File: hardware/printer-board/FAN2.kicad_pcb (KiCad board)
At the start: 2 copper layers, 8 parts, among them J35 TO FAN2, Q6 D882

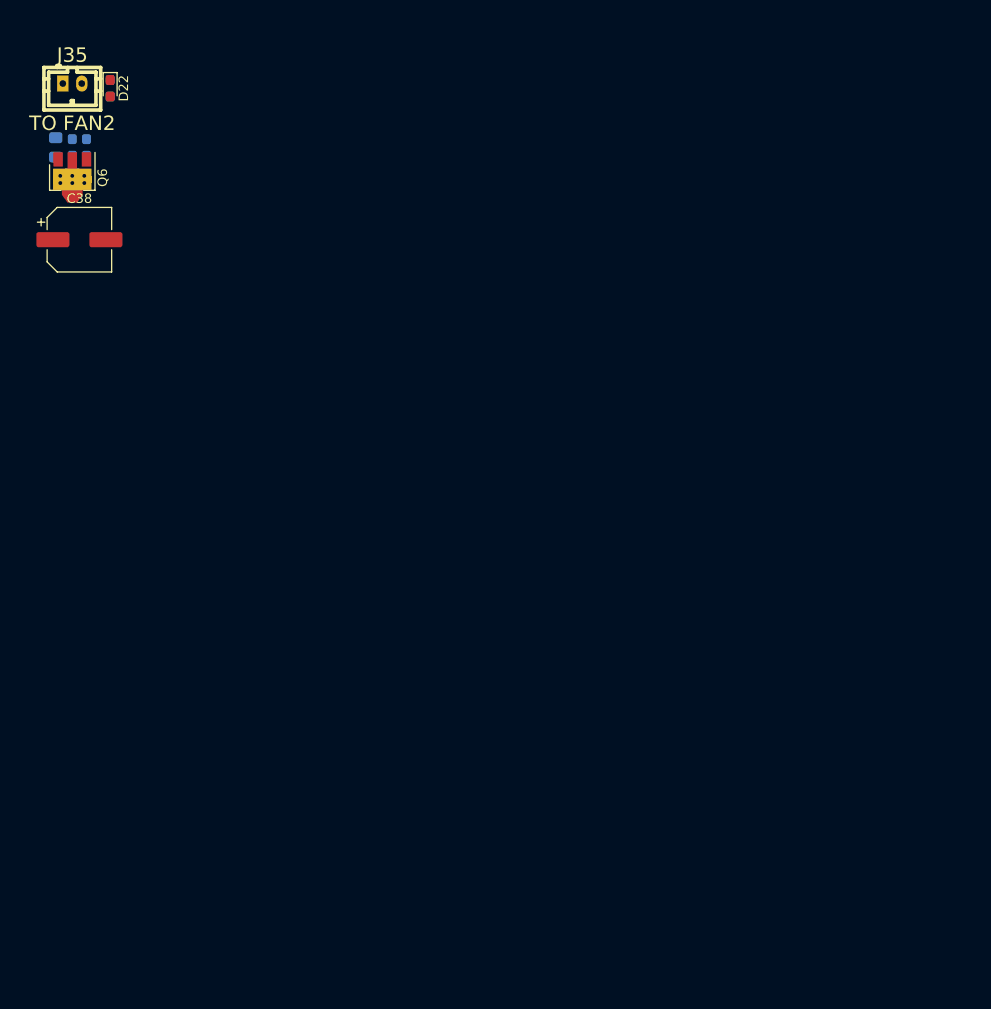
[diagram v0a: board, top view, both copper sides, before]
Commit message: update,
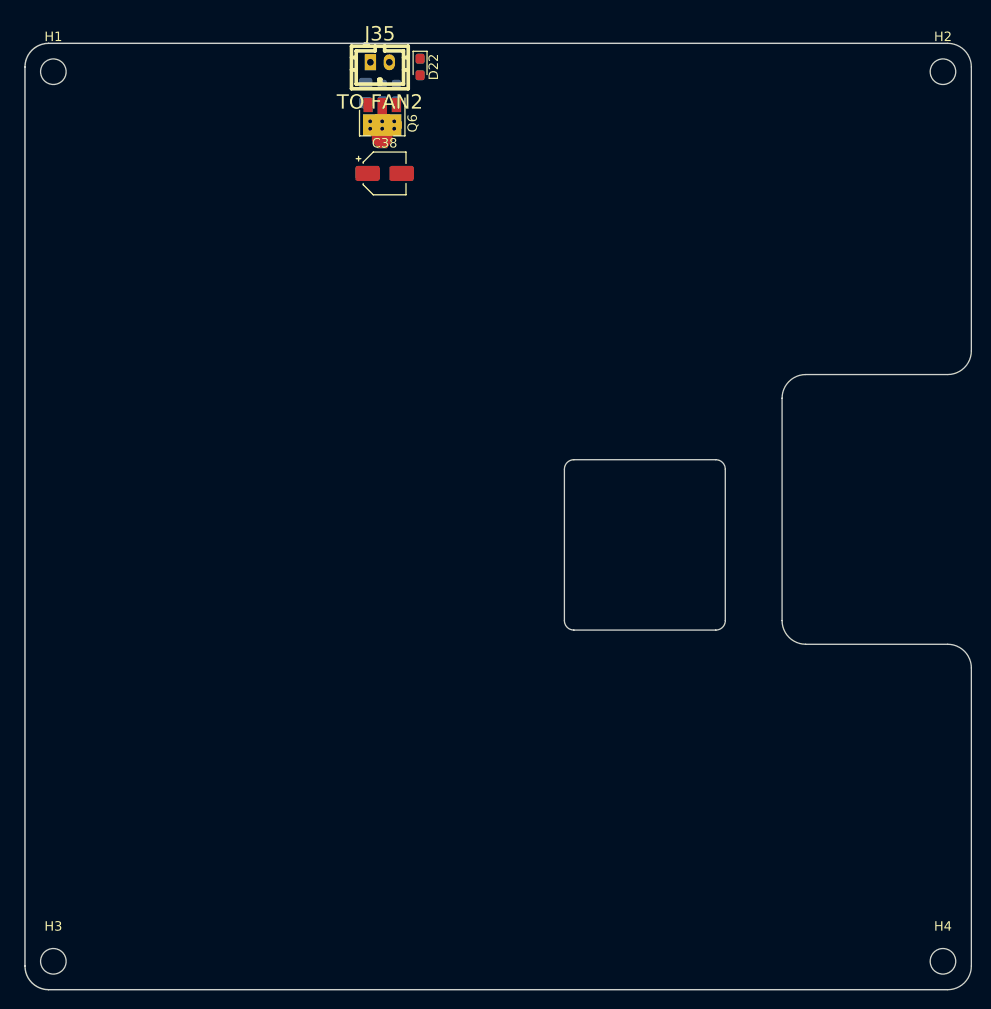
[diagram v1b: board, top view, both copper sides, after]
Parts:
- added H1: MOUNT_M3, MountingHole:MountingHole_2.7mm_M2.5, F.Cu at (3.00, 3.00)
- added H2: MOUNT_M3, MountingHole:MountingHole_2.7mm_M2.5, F.Cu at (97.0, 3.00)
- added H3: MOUNT_M3, MountingHole:MountingHole_2.7mm_M2.5, F.Cu at (3.00, 97.0)
- added H4: MOUNT_M3, MountingHole:MountingHole_2.7mm_M2.5, F.Cu at (97.0, 97.0)
- C38: value CP100uf,16V -> CP1uf,50V; footprint Capacitor_SMD:CP_Elec_6.3x5.3 -> Capacitor_SMD:CP_Elec_4x5.3
- moved Q6 33.3 mm to (37.8, 8.00)
- moved R64 33.3 mm to (39.2, 5.25)
- moved R65 33.3 mm to (36.0, 5.25)
- moved R66 33.3 mm to (37.8, 5.25)
- moved C38 33.0 mm to (38.0, 13.8)
- moved D22 32.8 mm to (41.8, 2.50)
- moved R67 32.8 mm to (41.8, 2.50)
- moved J35 32.6 mm to (37.5, 2.00)
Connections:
- C38 pad 2: GND -> Net-(C38-Pad2)
- D22 pad 1: Net-(D22-Pad1) -> Net-(C38-Pad2)
- J35 pad 2: Net-(D22-Pad1) -> Net-(C38-Pad2)
- R66 pad 1: Net-(D22-Pad1) -> Net-(C38-Pad2)
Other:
- board outline added: 100 x 100 mm
